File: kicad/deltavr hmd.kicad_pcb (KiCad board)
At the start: 2 copper layers, 38.7 x 48.5 mm, 10 parts, among them J1 Conn_02x07_Top_Bottom, U1 LSM6DSVTR, U2 nice_nano

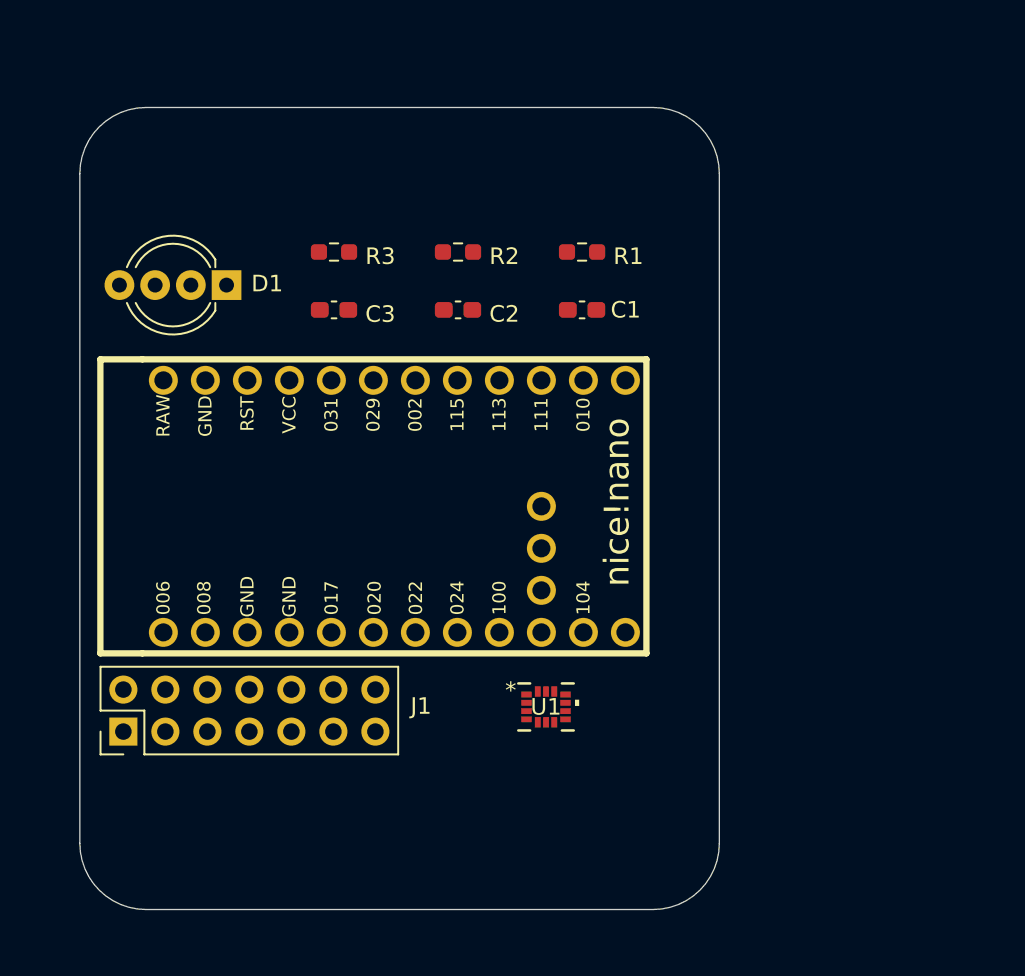
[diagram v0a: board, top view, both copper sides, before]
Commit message: kicad files after save for final pcb for hmd module
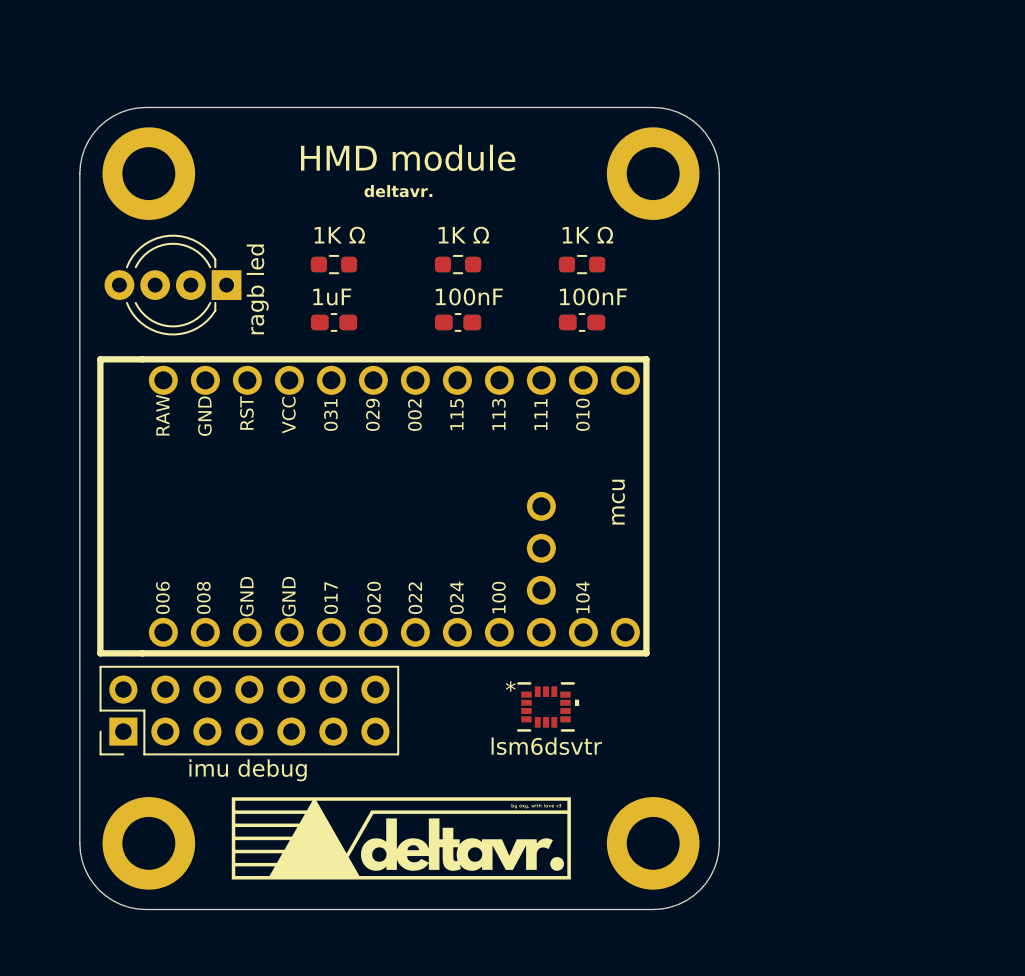
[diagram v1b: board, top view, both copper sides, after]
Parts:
- added M3 screw: MountingHole_3.2mm_M3_DIN965_Pad, MountingHole:MountingHole_3.2mm_M3_DIN965_Pad, F.Cu at (132.0, 83.5)
- added M3 screw: MountingHole_3.2mm_M3_DIN965_Pad, MountingHole:MountingHole_3.2mm_M3_DIN965_Pad, F.Cu at (132.0, 124.0)
- added M3 screw: MountingHole_3.2mm_M3_DIN965_Pad, MountingHole:MountingHole_3.2mm_M3_DIN965_Pad, F.Cu at (162.5, 124.0)
- added M3 screw: MountingHole_3.2mm_M3_DIN965_Pad, MountingHole:MountingHole_3.2mm_M3_DIN965_Pad, F.Cu at (162.5, 83.5)
- 1K Ω: renamed from R2
- 1K Ω: renamed from R1
- 1K Ω: renamed from R3
- imu debug: renamed from J1
- ragb led: renamed from D1
- moved 100nF 0.76 mm to (158.2, 92.5)
- moved 100nF 0.76 mm to (150.7, 92.5)
- moved 1K Ω 0.76 mm to (150.7, 89.0)
- moved 1K Ω 0.76 mm to (158.2, 89.0)
- moved 1K Ω 0.76 mm to (143.2, 89.0)
- moved 1uF 0.76 mm to (143.2, 92.5)
- renumbered C1 to 100nF, C2 to 100nF, C3 to 1uF, U1 to lsm6dsvtr
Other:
- board text added: "HMD module"
- board text added: "deltavr."

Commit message: hmd and controller done officially
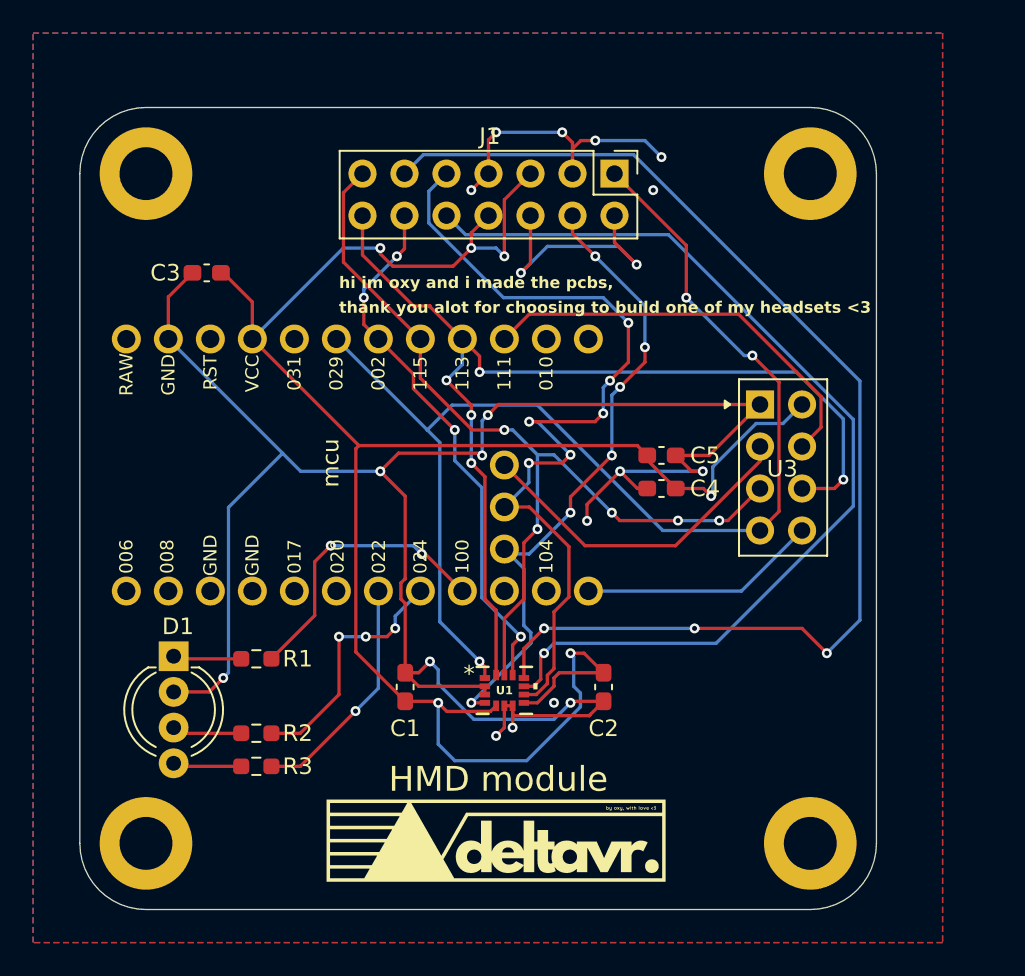
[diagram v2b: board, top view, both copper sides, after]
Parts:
- added C4: 10uF, Capacitor_SMD:C_0603_1608Metric_Pad1.08x0.95mm_HandSolder, F.Cu at (163.0, 102.5)
- added C5: 100nF, Capacitor_SMD:C_0603_1608Metric_Pad1.08x0.95mm_HandSolder, F.Cu at (163.0, 100.5)
- added U3: NRF24L01_Breakout, RF_Module:nRF24L01_Breakout, F.Cu at (169.0, 97.5)
- C3: renamed from 1uF; value 1uF -> 100nF
- D1: renamed from ragb led
- J1: renamed from imu debug
- R1, R2, R3: renamed from 1K Ω
- moved J1 44.9 mm to (160.2, 83.5), turned to -90 degrees
- moved R1 30.9 mm to (138.5, 112.8), turned to 0 degrees
- moved R2 30.9 mm to (138.5, 117.3), turned to 0 degrees
- moved R3 30.7 mm to (138.5, 119.3), turned to 0 degrees
- moved C1 24.5 mm to (147.5, 114.5), turned to -90 degrees
- moved C2 23.7 mm to (159.5, 114.5), turned to -90 degrees
- moved D1 22.7 mm to (133.5, 112.7), turned to -90 degrees
- moved M3 screw 9.50 mm to (172.0, 124.0)
- moved M3 screw 9.50 mm to (172.0, 83.5)
- moved C3 8.26 mm to (135.5, 89.5), turned to 180 degrees
- moved U2 3.36 mm to (144.6, 101.1)
- moved U1 2.71 mm to (153.5, 114.8)
- moved M3 screw 0.17 mm to (131.8, 83.5)
- moved M3 screw 0.17 mm to (131.8, 124.0)
- renumbered 100nF to C1, 100nF to C2, lsm6dsvtr to U1
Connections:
- net Net-(J1-Pin_14) renamed /sda
- C1 pad 1: Net-(J1-Pin_5) -> /gnd
- C1 pad 2: Net-(J1-Pin_2) -> /3.3v
- C2 pad 1: Net-(J1-Pin_2) -> /3.3v
- C2 pad 2: Net-(J1-Pin_5) -> /gnd
- C3 pad 1: Net-(J1-Pin_5) -> /3.3v
- C3 pad 2: Net-(J1-Pin_2) -> /gnd
- D1 pad 2: Net-(D1-A) -> /gnd
- J1 pad 1: Net-(J1-Pin_1) -> /sdo
- J1 pad 12: Net-(J1-Pin_12) -> /cs
- J1 pad 13: Net-(J1-Pin_13) -> /scl
- J1 pad 2: Net-(J1-Pin_2) -> /gnd
- J1 pad 3: Net-(J1-Pin_2) -> /gnd
- J1 pad 4: Net-(J1-Pin_4) -> /int1
- J1 pad 5: Net-(J1-Pin_5) -> /3.3v
- J1 pad 6: Net-(J1-Pin_2) -> /gnd
- J1 pad 7: Net-(J1-Pin_2) -> /gnd
- J1 pad 8: Net-(J1-Pin_5) -> /3.3v
- J1 pad 9: Net-(J1-Pin_9) -> /int2
- U1 pad 1: Net-(J1-Pin_1) -> /sdo
- U1 pad 12: Net-(J1-Pin_12) -> /cs
- U1 pad 13: Net-(J1-Pin_13) -> /scl
- U1 pad 2: Net-(J1-Pin_2) -> /gnd
- U1 pad 3: Net-(J1-Pin_2) -> /gnd
- U1 pad 4: Net-(J1-Pin_4) -> /int1
- U1 pad 5: Net-(J1-Pin_5) -> /3.3v
- U1 pad 6: Net-(J1-Pin_2) -> /gnd
- U1 pad 7: Net-(J1-Pin_2) -> /gnd
- U1 pad 8: Net-(J1-Pin_5) -> /3.3v
- U1 pad 9: Net-(J1-Pin_9) -> /int2
- U2 pad 12: unconnected-(U2-P1.06-Pad12) -> Net-(U2-P1.06)
- U2 pad 14: Net-(J1-Pin_12) -> unconnected-(U2-NFC2/P0.10-Pad14)
- U2 pad 15: Net-(J1-Pin_13) -> Net-(U2-P1.11)
- U2 pad 17: Net-(J1-Pin_1) -> /scl
- U2 pad 18: unconnected-(U2-AIN0/P0.02-Pad18) -> /cs
- U2 pad 19: unconnected-(U2-AIN5/P0.29-Pad19) -> /sdo
- U2 pad 21: Net-(J1-Pin_5) -> /3.3v
- U2 pad 23: unconnected-(U2-GND-Pad23) -> /gnd
- U2 pad 3: Net-(D1-A) -> unconnected-(U2-GND-Pad3)
- U2 pad 31: unconnected-(U2-P1.01-Pad31) -> /int1
- U2 pad 32: unconnected-(U2-P1.02-Pad32) -> /int2
- U2 pad 33: unconnected-(U2-P1.07-Pad33) -> Net-(U2-P1.07)
- U2 pad 4: Net-(J1-Pin_2) -> unconnected-(U2-GND-Pad4)
- U2 pad 5: Net-(J1-Pin_4) -> unconnected-(U2-P0.17-Pad5)
- U2 pad 6: Net-(J1-Pin_9) -> unconnected-(U2-P0.20-Pad6)
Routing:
- net /gnd: track 0.00 -> 160.4 mm, vias 0 -> 20
- net /3.3v: track 0.00 -> 119.9 mm, vias 0 -> 6
- net /sdo: track 0.00 -> 74.6 mm, vias 0 -> 3
- net Net-(J1-Pin_11): track 0.00 -> 72.2 mm, vias 0 -> 3
- net /sda: track 0.00 -> 64.5 mm, vias 0 -> 5
- net Net-(J1-Pin_10): track 0.00 -> 60.2 mm, vias 0 -> 1
- net /scl: track 0.00 -> 53.8 mm, vias 0 -> 5
- net /int2: track 0.00 -> 53.5 mm, vias 0 -> 6
- net /int1: track 0.00 -> 39.1 mm, vias 0 -> 6
- net /cs: track 0.00 -> 32.9 mm, vias 0 -> 4
- net Net-(U2-P1.11): track 0.00 -> 25.3 mm
- net Net-(U2-P1.07): track 0.00 -> 21.4 mm, vias 0 -> 1
- net Net-(U2-P1.00): track 0.00 -> 17.4 mm, vias 0 -> 2
- net Net-(U2-P0.24): track 0.00 -> 15.1 mm, vias 0 -> 3
- net Net-(U2-P1.06): track 0.00 -> 14.4 mm
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- added copper zone on B.Cu, net /gnd
- added copper zone on F.Cu, net /gnd
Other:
- board size 38.7 x 48.5 mm -> 48.2 x 48.5 mm
- board text added: "hi im oxy and i made the pcbs,"
- board text added: "thank you alot for choosing to build one of my headsets <3"
- board text removed: "deltavr."
